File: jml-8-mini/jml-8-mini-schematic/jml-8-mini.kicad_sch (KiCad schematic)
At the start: 10 parts, among them J6 Z80 Lines, U1 Z80CPU

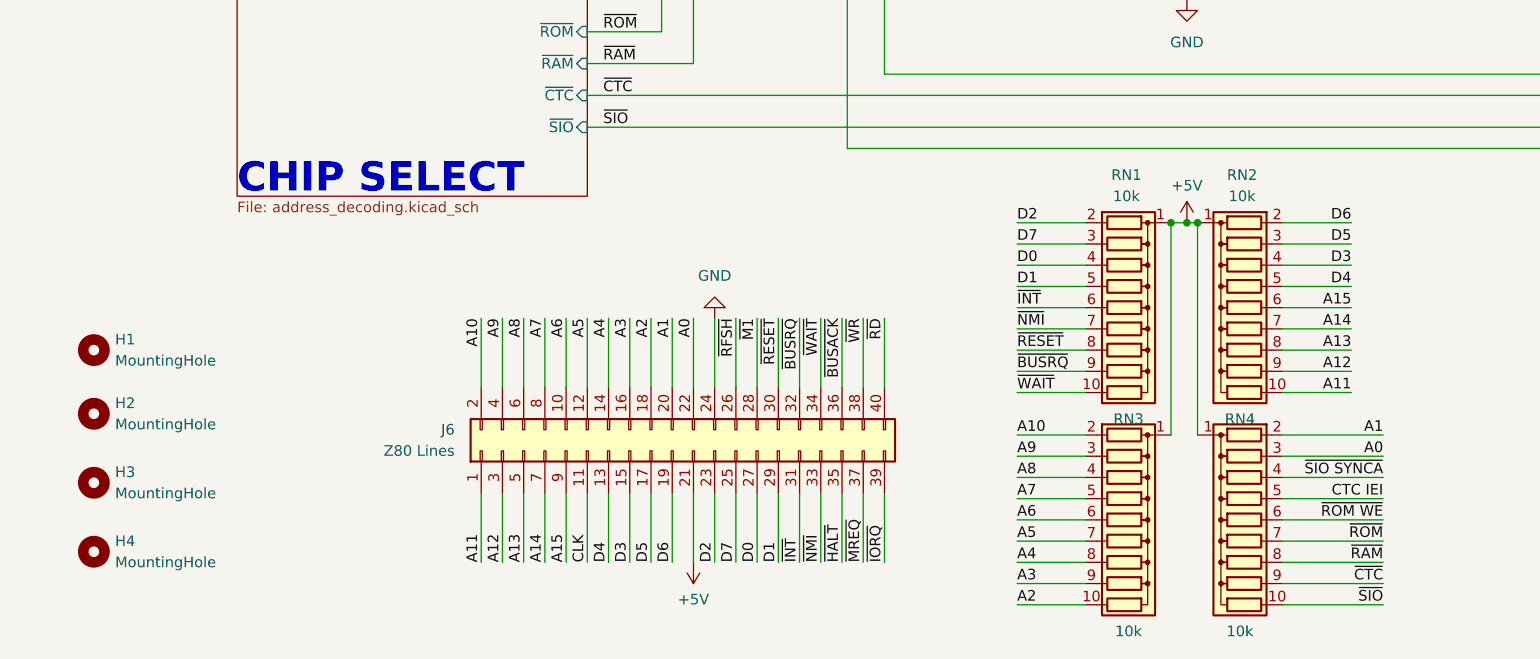
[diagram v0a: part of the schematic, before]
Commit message: lots of updates to schematic to make pcb routing easier, start on pcb design
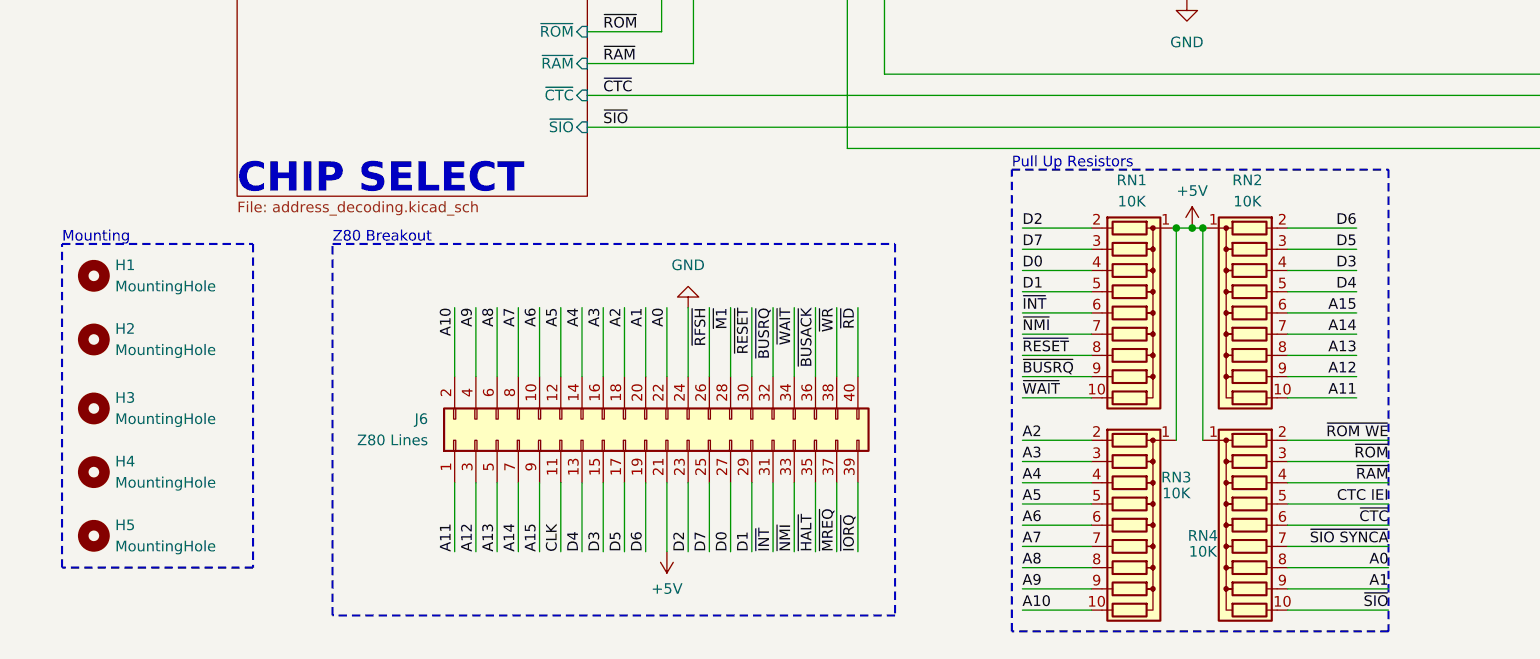
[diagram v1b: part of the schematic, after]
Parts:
- added H5: MountingHole, MountingHole:MountingHole_3.2mm_M3, symbol Mechanical:MountingHole
- H1, H2, H3, H4: footprint MountingHole:MountingHole_5mm -> MountingHole:MountingHole_3.2mm_M3
- RN1, RN2, RN3, RN4: value 10k -> 10K
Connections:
- net A0: now also RN4.8 (R7); no longer RN4.3 (R2)
- net A1: now also RN4.9 (R8); no longer RN4.2 (R1)
- net A10: now also RN3.10 (R9); no longer RN3.2 (R1)
- net A2: now also RN3.2 (R1); no longer RN3.10 (R9)
- net A3: now also RN3.3 (R2); no longer RN3.9 (R8)
- net A4: now also RN3.4 (R3); no longer RN3.8 (R7)
- net A5: now also RN3.5 (R4); no longer RN3.7 (R6)
- net A7: now also RN3.7 (R6); no longer RN3.5 (R4)
- net A8: now also RN3.8 (R7); no longer RN3.4 (R3)
- net A9: now also RN3.9 (R8); no longer RN3.3 (R2)
- net ~{CTC}: now also RN4.6 (R5); no longer RN4.9 (R8)
- net ~{RAM}: now also RN4.4 (R3); no longer RN4.8 (R7)
- net ~{ROM WE}: now also RN4.2 (R1); no longer RN4.6 (R5)
- net ~{ROM}: now also RN4.3 (R2); no longer RN4.7 (R6)
- net ~{SIO SYNCA}: now also RN4.7 (R6); no longer RN4.4 (R3)
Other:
- note added: "Mounting"
- note added: "Pull Up Resistors"
- note added: "Z80 Breakout"
- moved on the sheet: H1, H2, H3, J6, RN1, RN2, RN3, RN4
